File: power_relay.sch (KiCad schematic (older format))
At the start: 35 parts, among them J21 Conn_01x03, J22 Conn_01x03, J23 Conn_01x03, J24 Conn_01x03, J25 Conn_01x03, K1 lsts-devices:RELAY_1RT, K2 lsts-devices:RELAY_1RT, K3 lsts-devices:RELAY_1RT, K4 lsts-devices:RELAY_1RT, K5 lsts-devices:RELAY_1RT, Q12 MMBT4401-7-F, Q13 MMBT4401-7-F, Q14 MMBT4401-7-F, Q15 SI7113ADN-T1-GE3, Q16 SI7113ADN-T1-GE3, Q17 SI7113ADN-T1-GE3, Q18 MMBT4401-7-F, Q19 MMBT4401-7-F, Q20 SI7113ADN-T1-GE3, Q21 SI7113ADN-T1-GE3

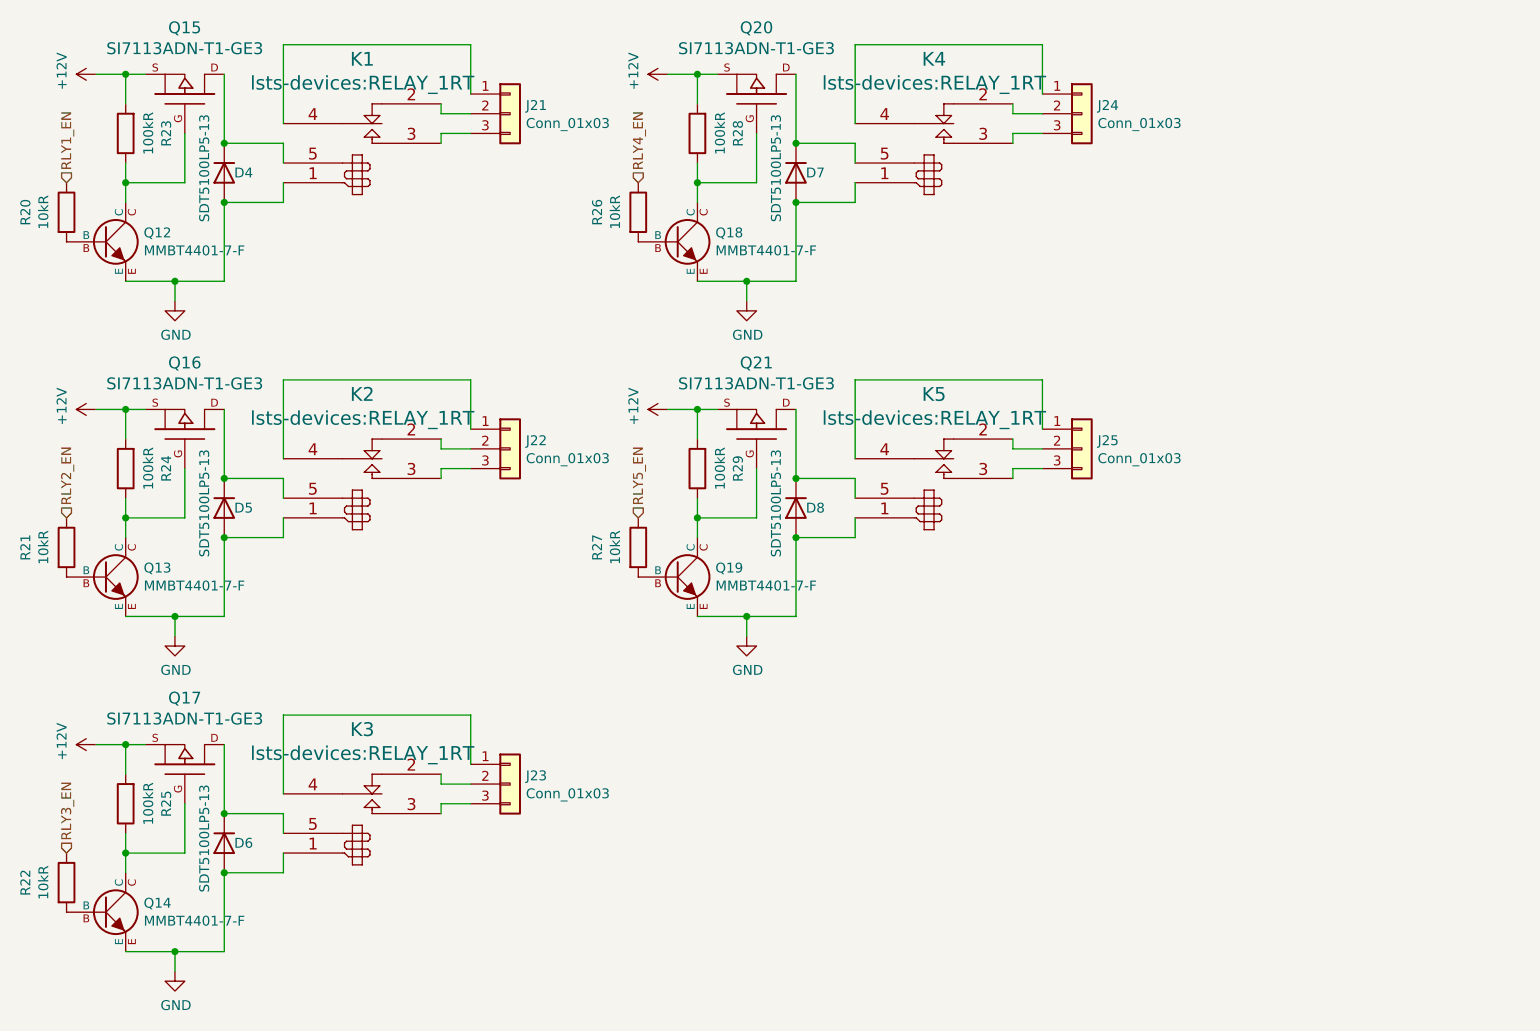
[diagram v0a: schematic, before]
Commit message: Final touches
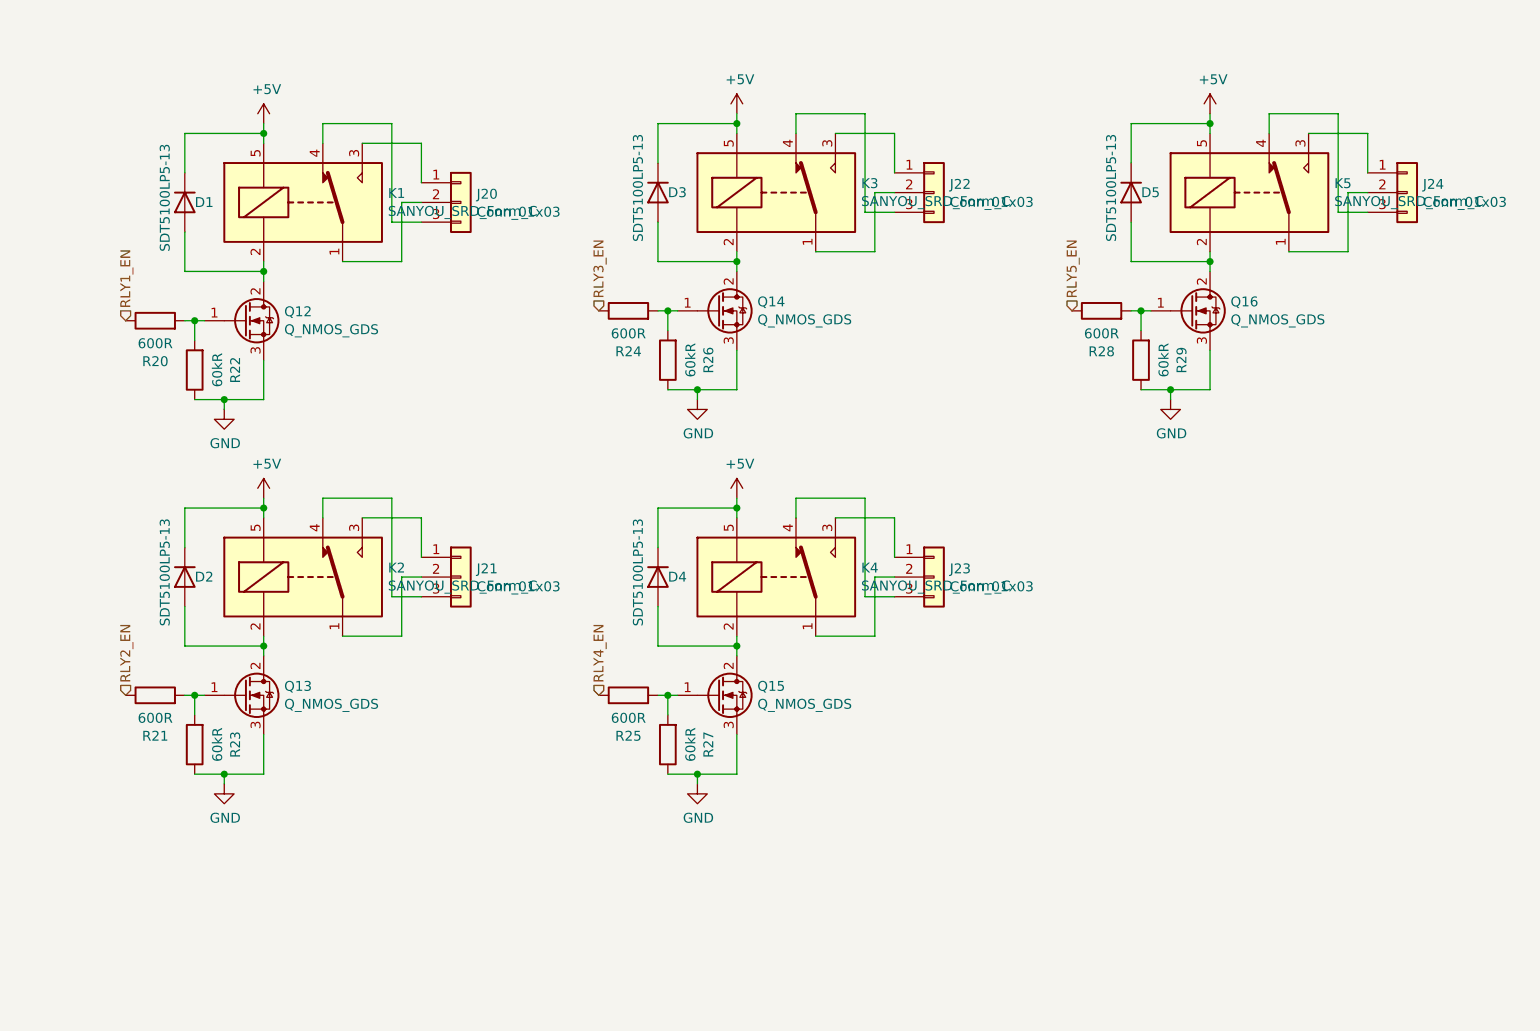
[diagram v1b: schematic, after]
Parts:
- removed D6, D7, D8: SDT5100LP5-13, Diode_SMD:D_PowerDI-5, symbol Device:D
- removed J25: Conn_01x03, TerminalBlock_Phoenix:TerminalBlock_Phoenix_PT-1,5-3-3.5-H_1x03_P3.50mm_Horizontal, symbol Connector_Generic:Conn_01x03
- removed K1, K2, K3, K4, K5: lsts-devices:RELAY_1RT, Relay_THT:Relay_SPDT_Panasonic_JW1_FormC_lsts, symbol lsts-devices:RELAY_1RT
- removed Q12, Q13, Q14, Q18, Q19: MMBT4401-7-F, lsts-discretes:SOT23_BC817, symbol lsts-discrete:NPN_EBC
- removed Q15, Q16, Q17, Q20, Q21: SI7113ADN-T1-GE3, lsts-discretes:PowerPAK_1212-8, symbol lsts-discrete:MOS_P
- added D1, D2, D3: SDT5100LP5-13, Diode_SMD:D_PowerDI-5, symbol Device:D
- added J20: Conn_01x03, TerminalBlock_Phoenix:TerminalBlock_Phoenix_PT-1,5-3-3.5-H_1x03_P3.50mm_Horizontal, symbol Connector_Generic:Conn_01x03
- added K1, K2, K3, K4, K5: SANYOU_SRD_Form_C, Relay_THT:Relay_SPDT_SANYOU_SRD_Series_Form_C, symbol Relay:SANYOU_SRD_Form_C
- added Q12, Q13, Q14, Q15, Q16: Q_NMOS_GDS, Package_TO_SOT_SMD:TO-252-2, symbol Device:Q_NMOS_GDS
- R20, R21: value 10kR -> 600R; footprint lsts-passives:R_0603 -> lsts_passives:R_0603; manf# CRCW060310K0JNEBC -> CRCW0603100KFKEAC
- R22, R26, R27: value 10kR -> 60kR; footprint lsts-passives:R_0603 -> lsts_passives:R_0603; manf# CRCW060310K0JNEBC -> CRCW0603100KFKEAC
- R23, R29: value 100kR -> 60kR; footprint lsts-passives:R_0603 -> lsts_passives:R_0603
- R24, R25, R28: value 100kR -> 600R; footprint lsts-passives:R_0603 -> lsts_passives:R_0603
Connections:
- net GND: now also R22.1, R23.1, R26.1, R27.1, R29.1, Q12.3 (S), Q13.3 (S), Q14.3 (S), Q15.3 (S), Q16.3 (S); no longer D4.2 (A), D5.2 (A)
- net RLY3_EN: now also R24.1; no longer R22.1
- net RLY4_EN: now also R25.1; no longer R26.1
- net RLY5_EN: now also R28.1; no longer R27.1
- net at R27.2: now also R25.2, Q15.1 (G)
- net at J24.2 (Pin_2): now also K5.1
- net at J24.3 (Pin_3): now also K5.4
- net at J24.1 (Pin_1): now also K5.3
- net at R26.2: now also R24.2, Q14.1 (G)
- net +5V: now reaches D5.1 (K)
- net +5V: now also D4.1 (K), D1.1 (K), D2.1 (K), D3.1 (K), K1.5, K2.5, K3.5, K4.5, K5.5
- net at J22.2 (Pin_2): now also K3.1
- net at J22.3 (Pin_3): now also K3.4
- net at J22.1 (Pin_1): now also K3.3
- net at R21.2: now also R23.2, Q13.1 (G)
- net at J21.2 (Pin_2): now also K2.1
- net at J21.3 (Pin_3): now also K2.4
- net at J21.1 (Pin_1): now also K2.3
- net at R20.2: now also R22.2, Q12.1 (G)
- net at J23.2 (Pin_2): now also K4.1
- net at J23.3 (Pin_3): now also K4.4
- net at J23.1 (Pin_1): now also K4.3
- removed net +12V: R23.2, R24.2, R25.2, R28.2, R29.2
- new net: J20.2 (Pin_2), K1.1
- new net: D1.2 (A), K1.2, Q12.2 (D)
- new net: J20.1 (Pin_1), K1.3
- new net: J20.3 (Pin_3), K1.4
- new net: D3.2 (A), K3.2, Q14.2 (D)
- new net: D5.2 (A), K5.2, Q16.2 (D)
- new net: Q16.1 (G), R28.2, R29.2
- new net: D2.2 (A), K2.2, Q13.2 (D)
- new net: D4.2 (A), K4.2, Q15.2 (D)
